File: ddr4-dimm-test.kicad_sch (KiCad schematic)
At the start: 137 parts, among them IC1 DDR4-BGA78, IC2 DDR4-BGA78, IC3 DDR4-BGA78, IC4 DDR4-BGA78, IC5 DDR4-BGA78, IC6 DDR4-BGA78, IC7 DDR4-BGA78, IC8 DDR4-BGA78

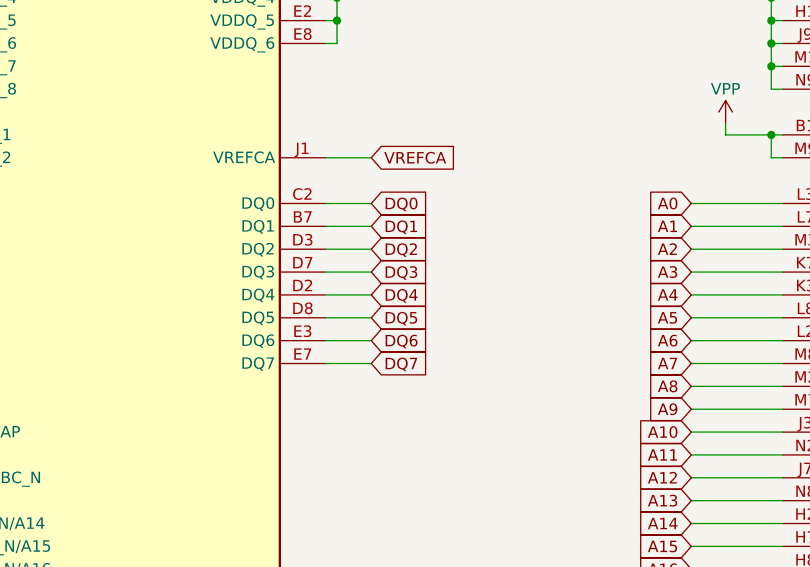
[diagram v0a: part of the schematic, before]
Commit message: Some more layout testing
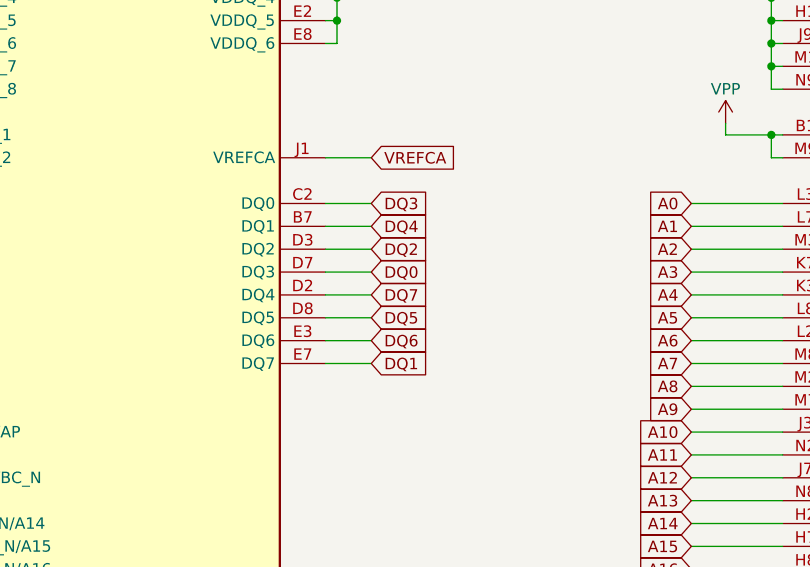
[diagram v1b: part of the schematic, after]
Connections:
- net DQ0: now also IC1.D7 (DQ3); no longer IC1.C2 (DQ0)
- net DQ1: now also IC1.E7 (DQ7); no longer IC1.B7 (DQ1)
- net DQ3: now also IC1.C2 (DQ0); no longer IC1.D7 (DQ3)
- net DQ4: now also IC1.B7 (DQ1); no longer IC1.D2 (DQ4)
- net DQ7: now also IC1.D2 (DQ4); no longer IC1.E7 (DQ7)
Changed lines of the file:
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@@
 	(global_label "DQ3"
 		(shape input)
-		(at 205.74 74.93 0)
+		(at 205.74 67.31 0)
 		(fields_autoplaced yes)
 		(effects
@@
 		)
 		(property "Intersheetrefs" "${INTERSHEET_REFS}"
-			(at 214.0471 74.93 0)
+			(at 214.0471 67.31 0)
 			(effects
 				(font
@@
 	(global_label "DQ1"
 		(shape input)
-		(at 205.74 69.85 0)
+		(at 205.74 85.09 0)
 		(fields_autoplaced yes)
 		(effects
@@
 		)
 		(property "Intersheetrefs" "${INTERSHEET_REFS}"
-			(at 214.0471 69.85 0)
+			(at 214.0471 85.09 0)
 			(effects
 				(font
@@
 	(global_label "DQ4"
 		(shape input)
-		(at 205.74 77.47 0)
+		(at 205.74 69.85 0)
 		(fields_autoplaced yes)
 		(effects
@@
 		)
 		(property "Intersheetrefs" "${INTERSHEET_REFS}"
-			(at 214.0471 77.47 0)
+			(at 214.0471 69.85 0)
 			(effects
 				(font
@@
 	(global_label "DQ7"
 		(shape input)
-		(at 205.74 85.09 0)
+		(at 205.74 77.47 0)
 		(fields_autoplaced yes)
 		(effects
@@
 		)
 		(property "Intersheetrefs" "${INTERSHEET_REFS}"
-			(at 214.0471 85.09 0)
+			(at 214.0471 77.47 0)
 			(effects
 				(font
@@
 	(global_label "DQ0"
 		(shape input)
-		(at 205.74 67.31 0)
+		(at 205.74 74.93 0)
 		(fields_autoplaced yes)
 		(effects
@@
 		)
 		(property "Intersheetrefs" "${INTERSHEET_REFS}"
-			(at 214.0471 67.31 0)
+			(at 214.0471 74.93 0)
 			(effects
 				(font
